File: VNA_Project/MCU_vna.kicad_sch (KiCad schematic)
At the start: 28 parts, among them J401 AVR-JTAG-10, SW401 SW_Push, SW402 SW_SPDT, U401 STM32H730VBTx, Y401 NX2016SA25MHz

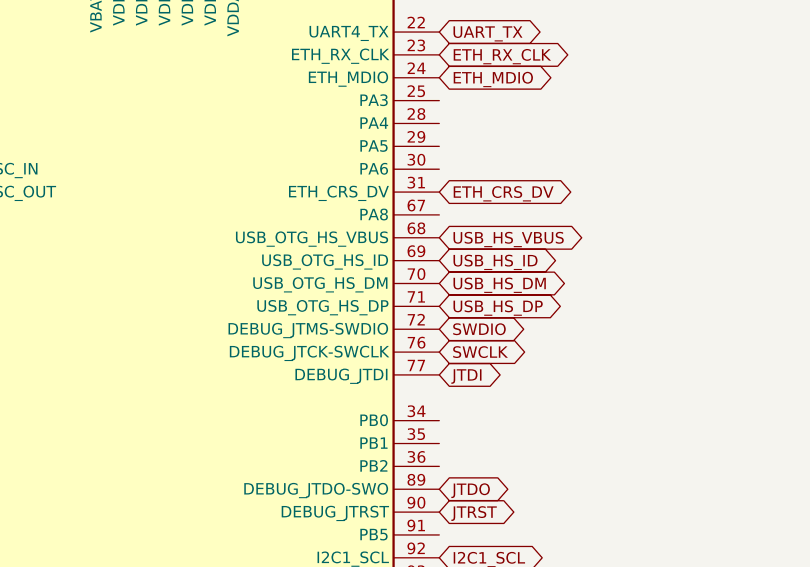
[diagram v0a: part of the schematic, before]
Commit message: minor changes
minor changes
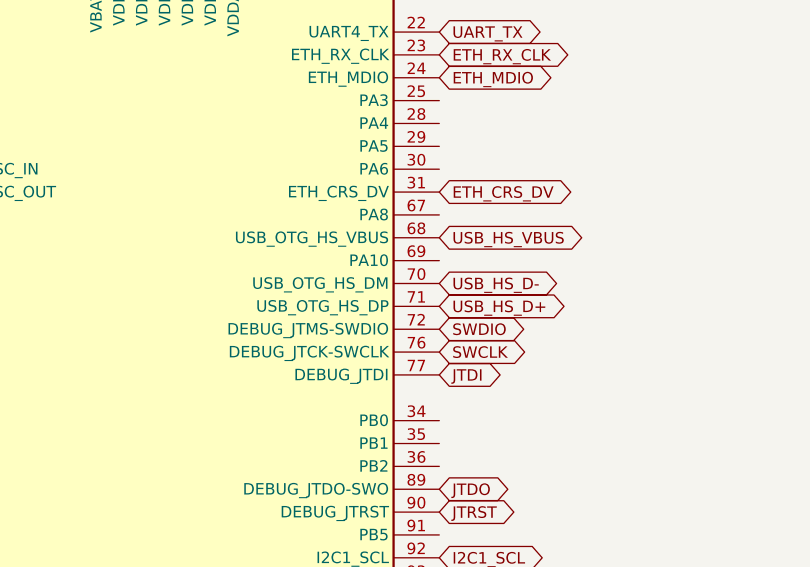
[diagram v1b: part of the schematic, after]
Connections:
- net USB_HS_DM renamed USB_HS_D-
- net USB_HS_DP renamed USB_HS_D+
- net USB_HS_ID: no longer names the net of U401.69 (PA10)

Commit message: minor changes
minor changes
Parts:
- removed D403: ESDA6V1SC5, Package_TO_SOT_SMD:SOT-23-5, symbol Power_Protection:ESDA6V1SC5
- removed J401: AVR-JTAG-10, symbol Connector:AVR-JTAG-10
- added C18: 100nF, Capacitor_SMD:C_0402_1005Metric, symbol Device:C
- added D403, D404, D405, D406, D407, D408, D409, D410: ESD131-B1-W0201, Diode_SMD:Infineon_SG-WLL-2-3_0.58x0.28_P0.36mm, symbol Diode:ESD131-B1-W0201
- added FB401: FerriteBead, symbol Device:FerriteBead
- added J2: SWD TC2030, Connector:Tag-Connect_TC2030-IDC-FP_2x03_P1.27mm_Vertical, symbol Connector:Conn_ARM_SWD_TagConnect_TC2030
- added J401, J402: Conn_01x04_Pin, symbol Connector:Conn_01x04_Pin
- added J403, J5: Conn_01x04_Pin, Connector_PinSocket_2.00mm:PinSocket_1x04_P2.00mm_Vertical, symbol Connector:Conn_01x04_Pin
- added R405, R406, R8, R9: 1.5K, Resistor_SMD:R_0402_1005Metric, symbol Device:R
- added R5, R6: 220R, Resistor_SMD:R_0402_1005Metric, symbol Device:R
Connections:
- net +3.3V: now also J2.1 (VCC), J401.1 (Pin_1), J402.1 (Pin_1), J403.1 (Pin_1), J5.1 (Pin_1), R405.1, R406.1, R8.1, R9.1
- net +3.3VA: now also FB401.2; no longer C409.1, C410.1, U401.21 (VDDA)
- net GND: now also C18.1, D403.1 (A1), D404.1 (A1), D405.1 (A1), D406.1 (A1), D407.1 (A1), D408.1 (A1), D409.1 (A1), D410.1 (A1), J2.5 (GND), J401.4 (Pin_4), J402.4 (Pin_4), J403.4 (Pin_4), J5.4 (Pin_4)
- net I2C1_SCL: now also D407.2 (A2), J5.2 (Pin_2), R8.2
- net I2C1_SDA: now also D408.2 (A2), J5.3 (Pin_3), R9.2
- net I2C4_SCL: now also D409.2 (A2), J403.2 (Pin_2), R405.2
- net I2C4_SDA: now also D410.2 (A2), J403.3 (Pin_3), R406.2
- net JTDO: now also J2.6 (SWO)
- net NRST: now also C18.2, J2.3 (~{RESET})
- net SWCLK: now also D405.2 (A2), J2.2 (SWDIO), J402.3 (Pin_3)
- net SWDIO: now also D404.2 (A2), J2.4 (SWCLK), J402.2 (Pin_2)
- net UART_RX: now also D406.2 (A2), R6.2
- net UART_TX: now also R5.2
- net vref+: now reaches R401.2, U401.20 (VREF+)
- new net: D403.2 (A2), J401.2 (Pin_2), R5.1
- new net: J401.3 (Pin_3), R6.1
- new net analog decoupling: C409.1, C410.1, FB401.1, U401.21 (VDDA)
- no-connect marks 2 -> 1
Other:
- note added: "2 - I2C4"
- note added: "I2C1"
- note added: "SWD"
- note added: "SWD 2"
- note added: "UART"
- note removed: "JTAG/SWD"
- moved on the sheet: C409, C410

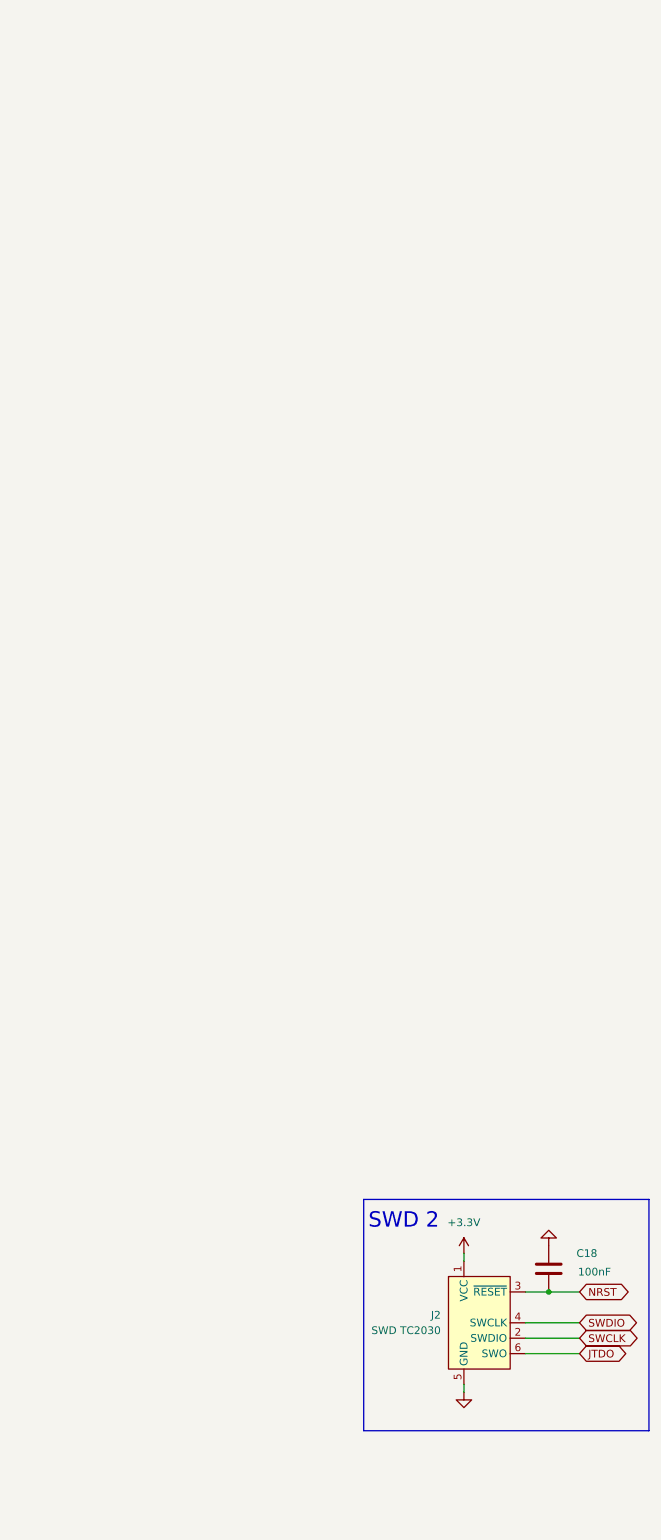
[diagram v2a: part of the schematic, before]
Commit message: minor changes eth
minor changes eth
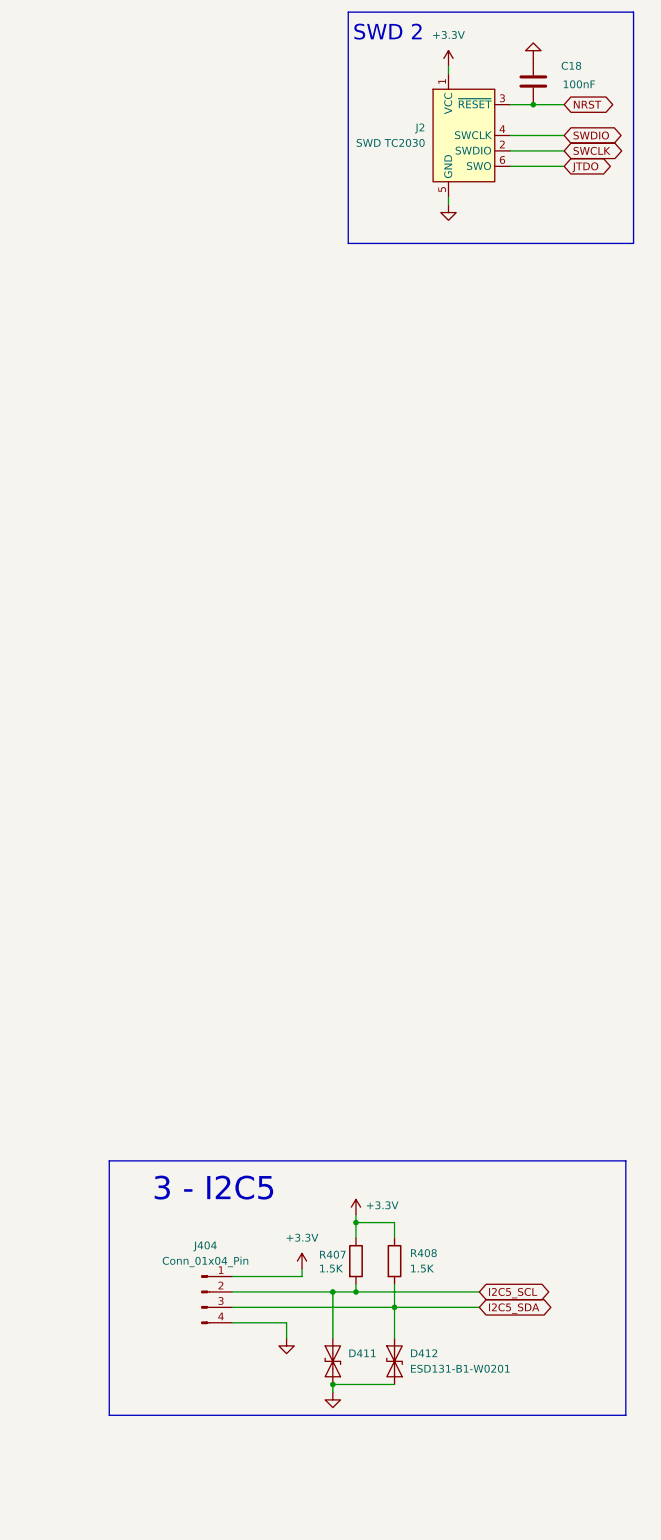
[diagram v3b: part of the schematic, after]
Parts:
- added D411, D412: ESD131-B1-W0201, Diode_SMD:Infineon_SG-WLL-2-3_0.58x0.28_P0.36mm, symbol Diode:ESD131-B1-W0201
- added J404: Conn_01x04_Pin, Connector_PinSocket_2.00mm:PinSocket_1x04_P2.00mm_Vertical, symbol Connector:Conn_01x04_Pin
- added R407, R408: 1.5K, Resistor_SMD:R_0402_1005Metric, symbol Device:R
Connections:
- net +3.3V: now also J404.1 (Pin_1), R407.1, R408.1
- net GND: now also D411.1 (A1), D412.1 (A1), J404.4 (Pin_4)
- net I2C5_SCL: now also D411.2 (A2), J404.2 (Pin_2), R407.2
- net I2C5_SDA: now also D412.2 (A2), J404.3 (Pin_3), R408.2
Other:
- note added: "3 - I2C5"
- moved on the sheet: C18, J2
